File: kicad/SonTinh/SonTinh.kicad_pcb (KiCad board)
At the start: 2 copper layers, 111.2 x 81 mm, 14 parts, among them J10 1985195, J11 Conn_01x03_Socket, J12 1985195, J13 Conn_01x03_Socket, J4 1985218, J5 1985218, J7 1985195, J8 1985195

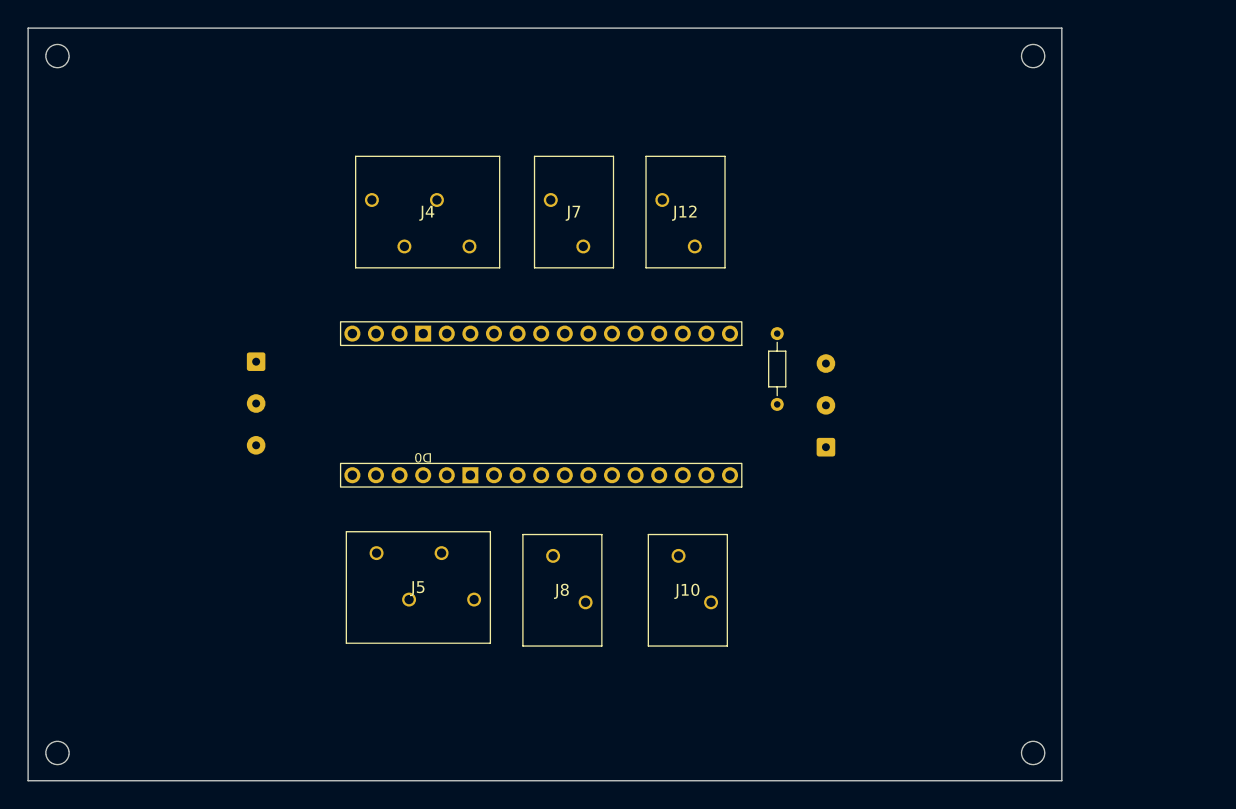
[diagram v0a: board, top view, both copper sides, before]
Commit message: The Quill Is Mightier…
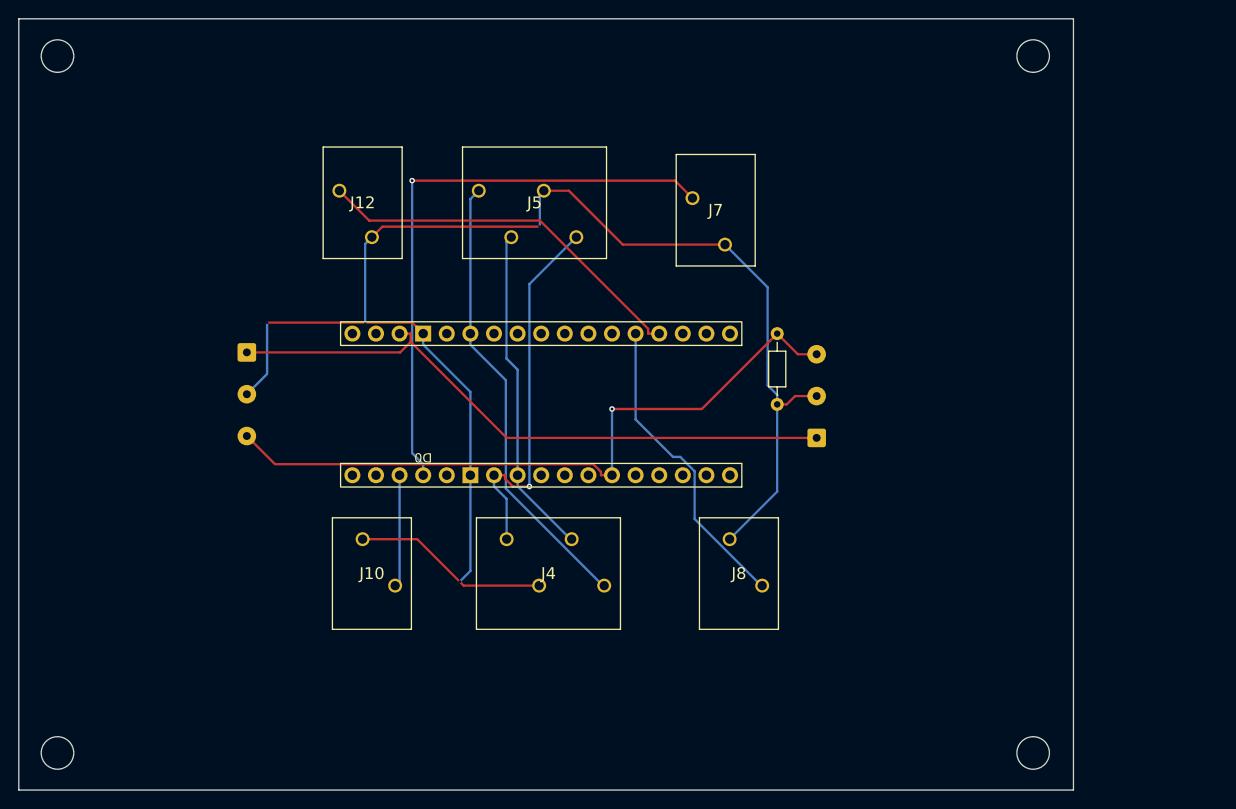
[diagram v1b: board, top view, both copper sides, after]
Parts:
- removed H1, H2, H3, H4: MountingHole_2.5mm, MountingHole:MountingHole_2.5mm
- added M1: MountingHole_3.5mm, MountingHole:MountingHole_3.5mm, F.Cu at (35.5, 95.5)
- added M2: MountingHole_3.5mm, MountingHole:MountingHole_3.5mm, F.Cu at (140.5, 95.5)
- added M3: MountingHole_3.5mm, MountingHole:MountingHole_3.5mm, F.Cu at (140.5, 20.5)
- added M4: MountingHole_3.5mm, MountingHole:MountingHole_3.5mm, F.Cu at (35.5, 20.5)
- moved J5 40.2 mm to (91.3, 40.0), turned to 180 degrees
- moved J12 34.8 mm to (72.6, 40.0)
- moved J10 34.0 mm to (65.1, 72.5)
- moved J4 31.8 mm to (83.8, 72.5), turned to 0 degrees
- moved J8 19.1 mm to (104.6, 72.5)
- moved J7 15.3 mm to (110.6, 40.8)
- moved J11 1.41 mm to (55.9, 52.4)
- moved J13 1.41 mm to (117.2, 61.6)
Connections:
- A1 pad A2: /A2 -> unconnected-(A1-PadA2)
- A1 pad A3: /A3 -> unconnected-(A1-PadA3)
- A1 pad A4: /A4 -> unconnected-(A1-PadA4)
- A1 pad A5: /A5 -> unconnected-(A1-PadA5)
- A1 pad D10: /A10 -> unconnected-(A1-PadD10)
- A1 pad D11: /D11 -> unconnected-(A1-PadD11)
- A1 pad D12: /A11 -> unconnected-(A1-PadD12)
- A1 pad D13: /D13 -> unconnected-(A1-PadD13)
- A1 pad D9: /D9 -> unconnected-(A1-PadD9)
- J11 pad 3: /D11 -> /D7
- J13 pad 3: /D11 -> /D7
- R13 pad 1: /D11 -> /D7
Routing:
- net GND: track 0.00 -> 171.0 mm, vias 0 -> 4
- net /D7: track 0.00 -> 74.7 mm, vias 0 -> 1
- net +12V: track 0.00 -> 68.2 mm
- net /D0: track 0.00 -> 63.1 mm, vias 0 -> 1
- net /5V: track 0.00 -> 48.9 mm
- net /A0: track 0.00 -> 41.1 mm
- net /SDA: track 0.00 -> 40.9 mm, vias 0 -> 1
- net /SCL: track 0.00 -> 35.7 mm
- net /A1: track 0.00 -> 33.3 mm
- net /D1: track 0.00 -> 12.1 mm
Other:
- board size 111.2 x 81 mm -> 113.5 x 83 mm

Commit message: The Bitter Suite
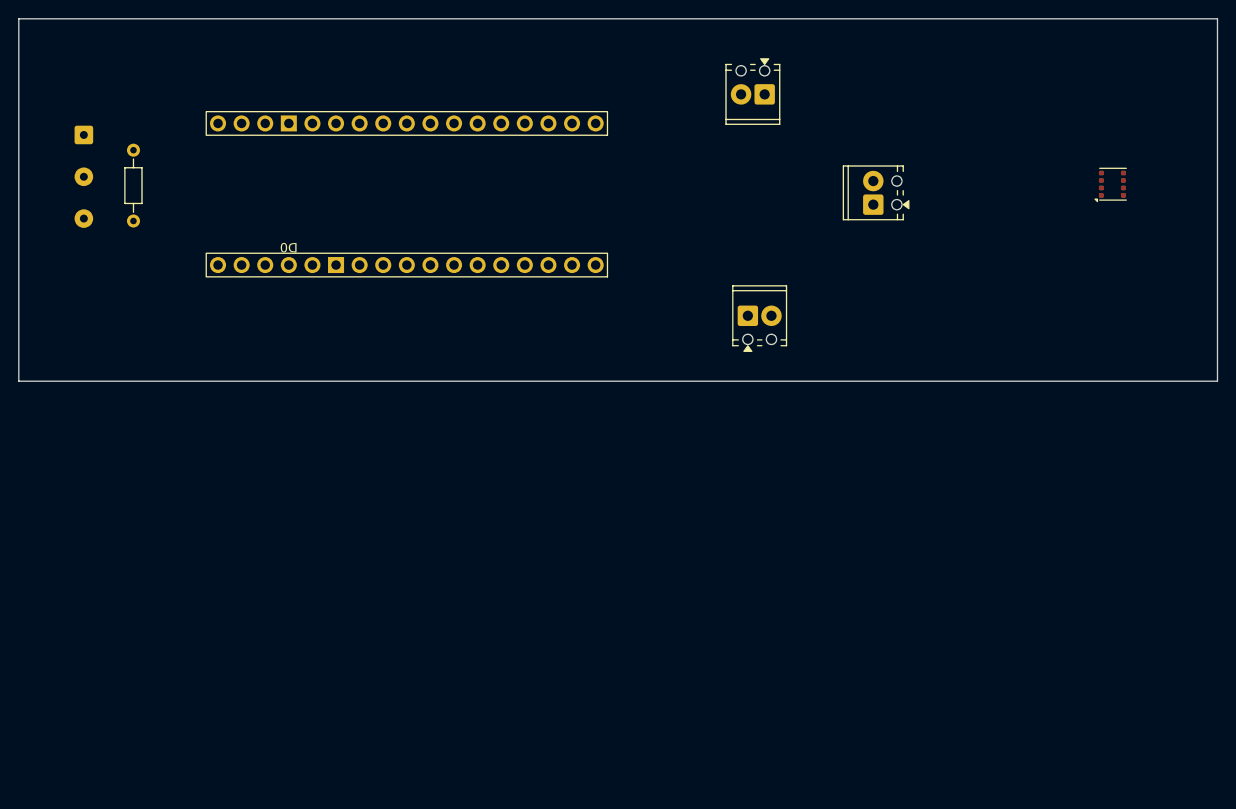
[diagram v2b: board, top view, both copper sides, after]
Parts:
- removed J10, J12, J7, J8: 1985195, footprints:1985195
- removed J13: Conn_01x03_Socket, Connector_Wire:SolderWire-0.25sqmm_1x03_P4.5mm_D0.65mm_OD2mm
- removed J4, J5: 1985218, footprints:PTSA_15_4_35_Z
- removed M1, M2, M3, M4: MountingHole_3.5mm, MountingHole:MountingHole_3.5mm
- added J1: Screw_Terminal_01x02, TerminalBlock_Phoenix:TerminalBlock_Phoenix_MPT-0,5-2-2.54_1x02_P2.54mm_Horizontal, F.Cu at (109.8, 48.5)
- added J2: Screw_Terminal_01x02, TerminalBlock_Phoenix:TerminalBlock_Phoenix_MPT-0,5-2-2.54_1x02_P2.54mm_Horizontal, F.Cu at (111.6, 24.6)
- added J3: Screw_Terminal_01x02, TerminalBlock_Phoenix:TerminalBlock_Phoenix_MPT-0,5-2-2.54_1x02_P2.54mm_Horizontal, F.Cu at (123.3, 36.5)
- added U1: BME680, Package_LGA:Bosch_LGA-8_3x3mm_P0.8mm_ClockwisePinNumbering, F.Cu at (149.0, 34.3)
- moved R13 70.3 mm to (43.7, 38.3), turned to 90 degrees
- moved J11 29.2 mm to (38.3, 29.0)
- moved A1 26.8 mm to (97.3, 26.4)
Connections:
- A1 pad MISO: unconnected-(A1-SPI_MISO-PadMISO) -> Net-(A1-SPI_MISO)
- A1 pad MOSI: unconnected-(A1-SPI_MOSI-PadMOSI) -> Net-(A1-SPI_MOSI)
- A1 pad SCK: unconnected-(A1-SPI_SCK-PadSCK) -> Net-(A1-SPI_SCK)
- A1 pad SS: unconnected-(A1-SPI_CS-PadSS) -> Net-(A1-SPI_CS)
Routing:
- net GND: track 171.0 -> 0.00 mm, vias 4 -> 0
- net /D7: track 74.7 -> 0.00 mm, vias 1 -> 0
- net +12V: track 68.2 -> 0.00 mm
- net /D0: track 63.1 -> 0.00 mm, vias 1 -> 0
- net /5V: track 48.9 -> 0.00 mm
- net /A0: track 41.1 -> 0.00 mm
- net /SDA: track 40.9 -> 0.00 mm, vias 1 -> 0
- net /SCL: track 35.7 -> 0.00 mm
- net /A1: track 33.3 -> 0.00 mm
- net /D1: track 12.1 -> 0.00 mm
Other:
- board size 113.5 x 83 mm -> 129 x 39 mm
